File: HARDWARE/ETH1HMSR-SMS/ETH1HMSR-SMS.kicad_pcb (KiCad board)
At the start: 4 copper layers, 100 x 45 mm, 126 parts, among them J201 1715721, J301 RJ45_Wuerth_7499010121A, J401 20021111-00010T4LF, J501 1710072, Q201 SI5618A, Q202 MMBT3904, U201 TSR_1-2450, U202 TLV62568DBV, U301 LAN8742A, U401 LT6350xMS8, U402 REF1933AIDDCT, U403 STM32H743VITx, U404 24LC08B-E/MS, U501 HMSR-SMS, U502 OPA4340UA, U503 DG412LEDQ, U504 DG419LEDY, Y301 NX5032GA-25, Y401 NX5032GA-16

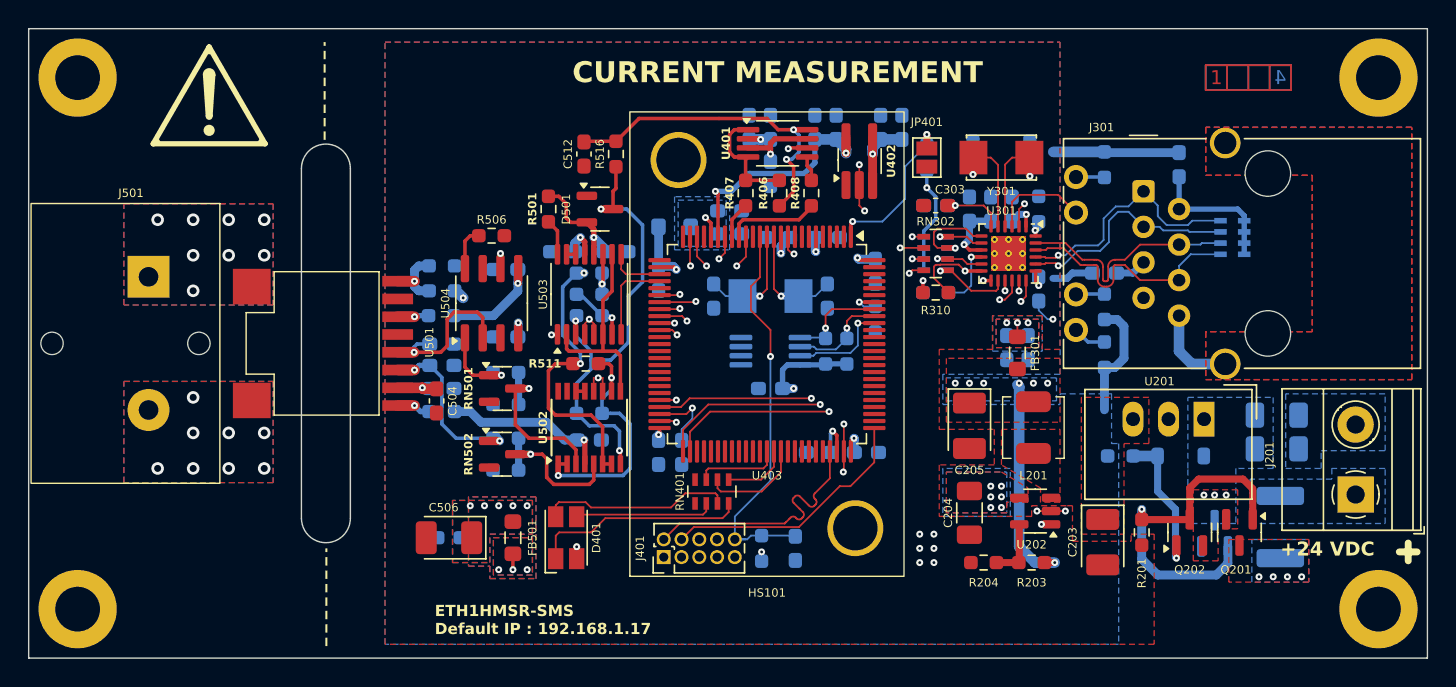
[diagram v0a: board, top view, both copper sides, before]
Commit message: development
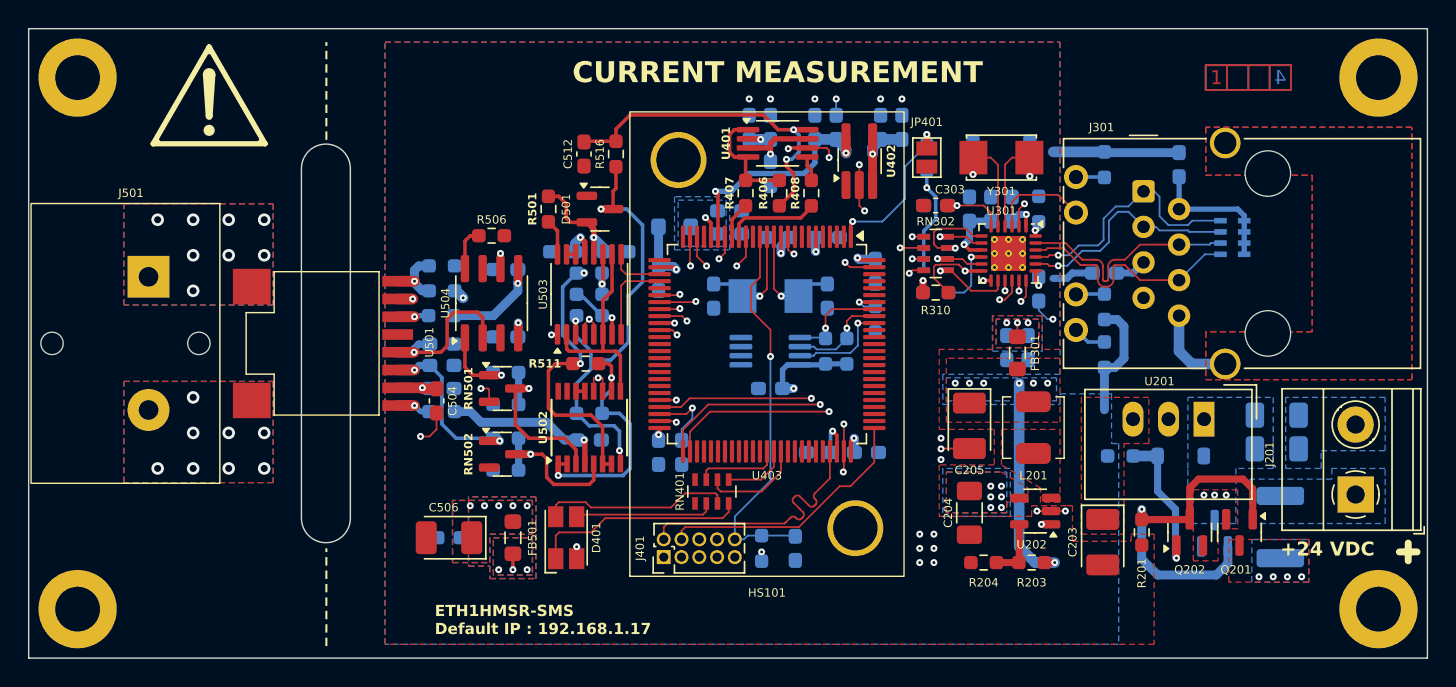
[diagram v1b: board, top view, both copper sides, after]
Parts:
- C512: value 100p -> DNP
- D501: value BAV99 -> BAV199
- R406, R512: value 0 -> DNP
- R516: value 100 -> 0
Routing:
- net GND: track 42.4 -> 55.1 mm, vias 19 -> 33
- net /MCU/NRST: track 48.2 -> 47.4 mm
- net /Current/VOUT: track 23.8 -> 24.5 mm
- net /Ethernet/ETH_RXN: track 18.1 -> 17.5 mm
- net /MCU/TMS_SWDIO: track 18.7 -> 19.3 mm

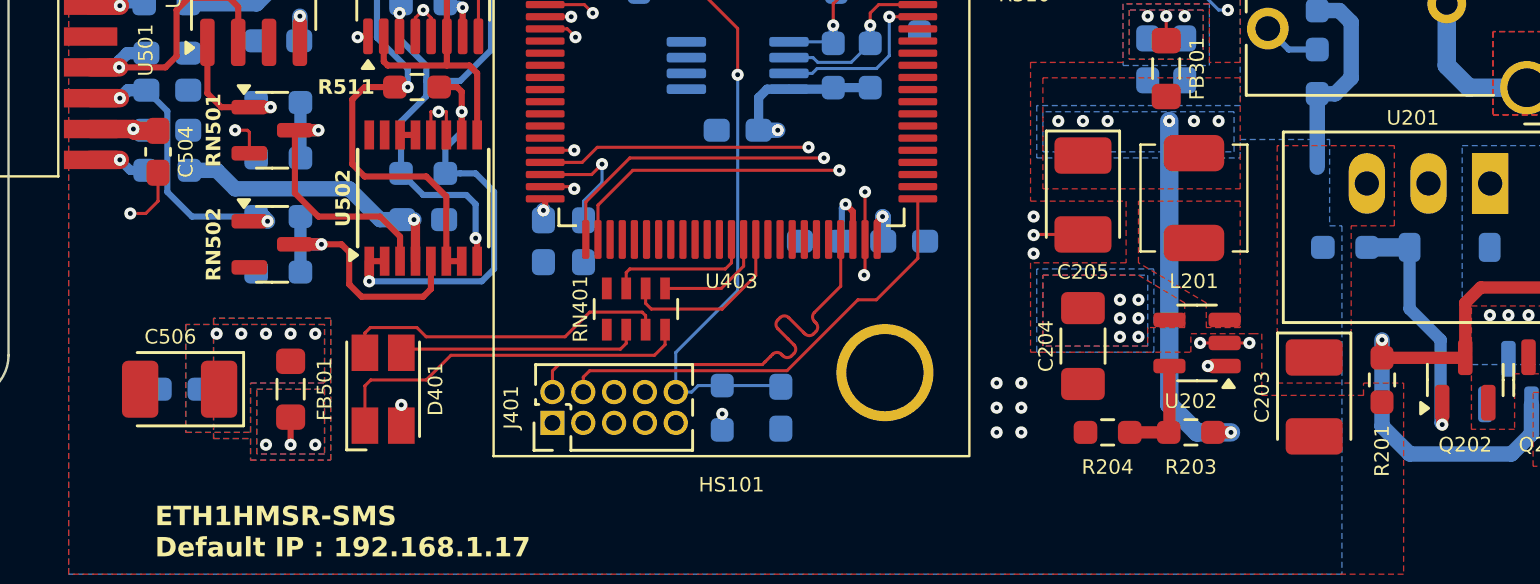
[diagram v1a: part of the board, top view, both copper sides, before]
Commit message: Development
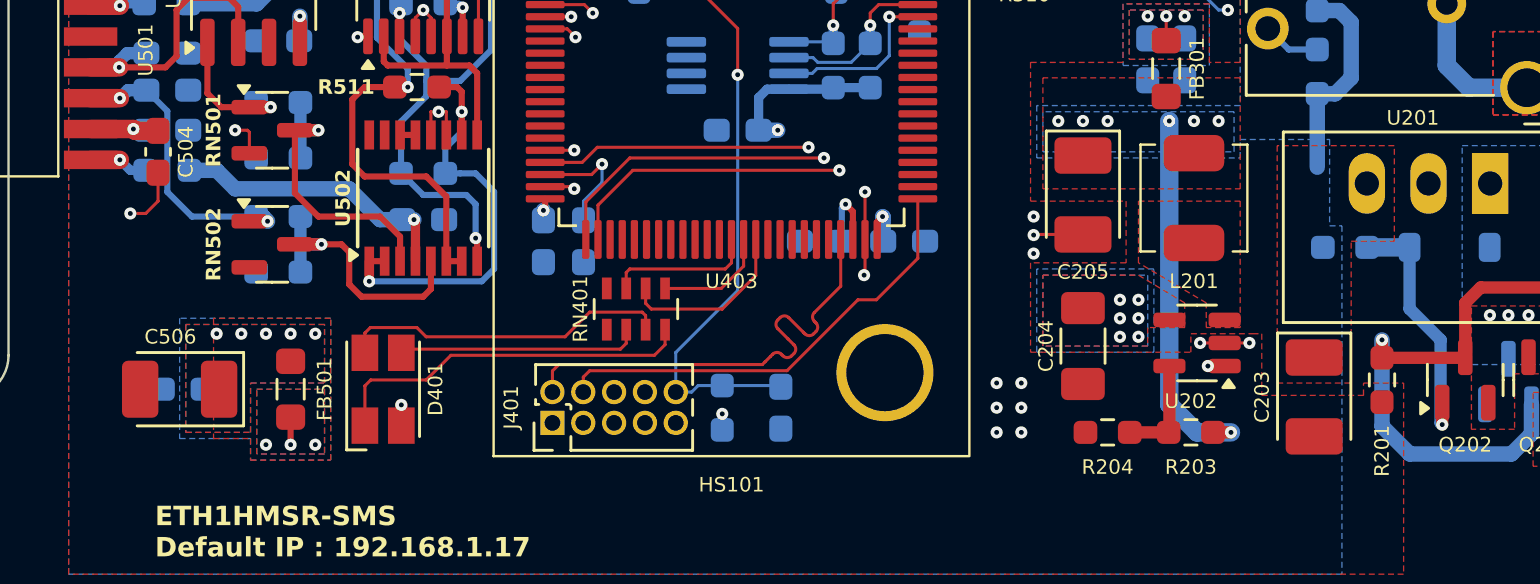
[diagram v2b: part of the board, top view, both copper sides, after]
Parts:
- moved C503 0.13 mm to (130.2, 96.4)
